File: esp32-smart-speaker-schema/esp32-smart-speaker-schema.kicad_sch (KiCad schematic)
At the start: 19 parts, among them J1 USB_C_Receptacle_USB2.0_14P, SW1 PWR_BTN, SW2 MODE_BTN, SW3 PREV_BTN, SW4 NXT_BTN, SW5 PAUS-BTN, U2 MAX98357A

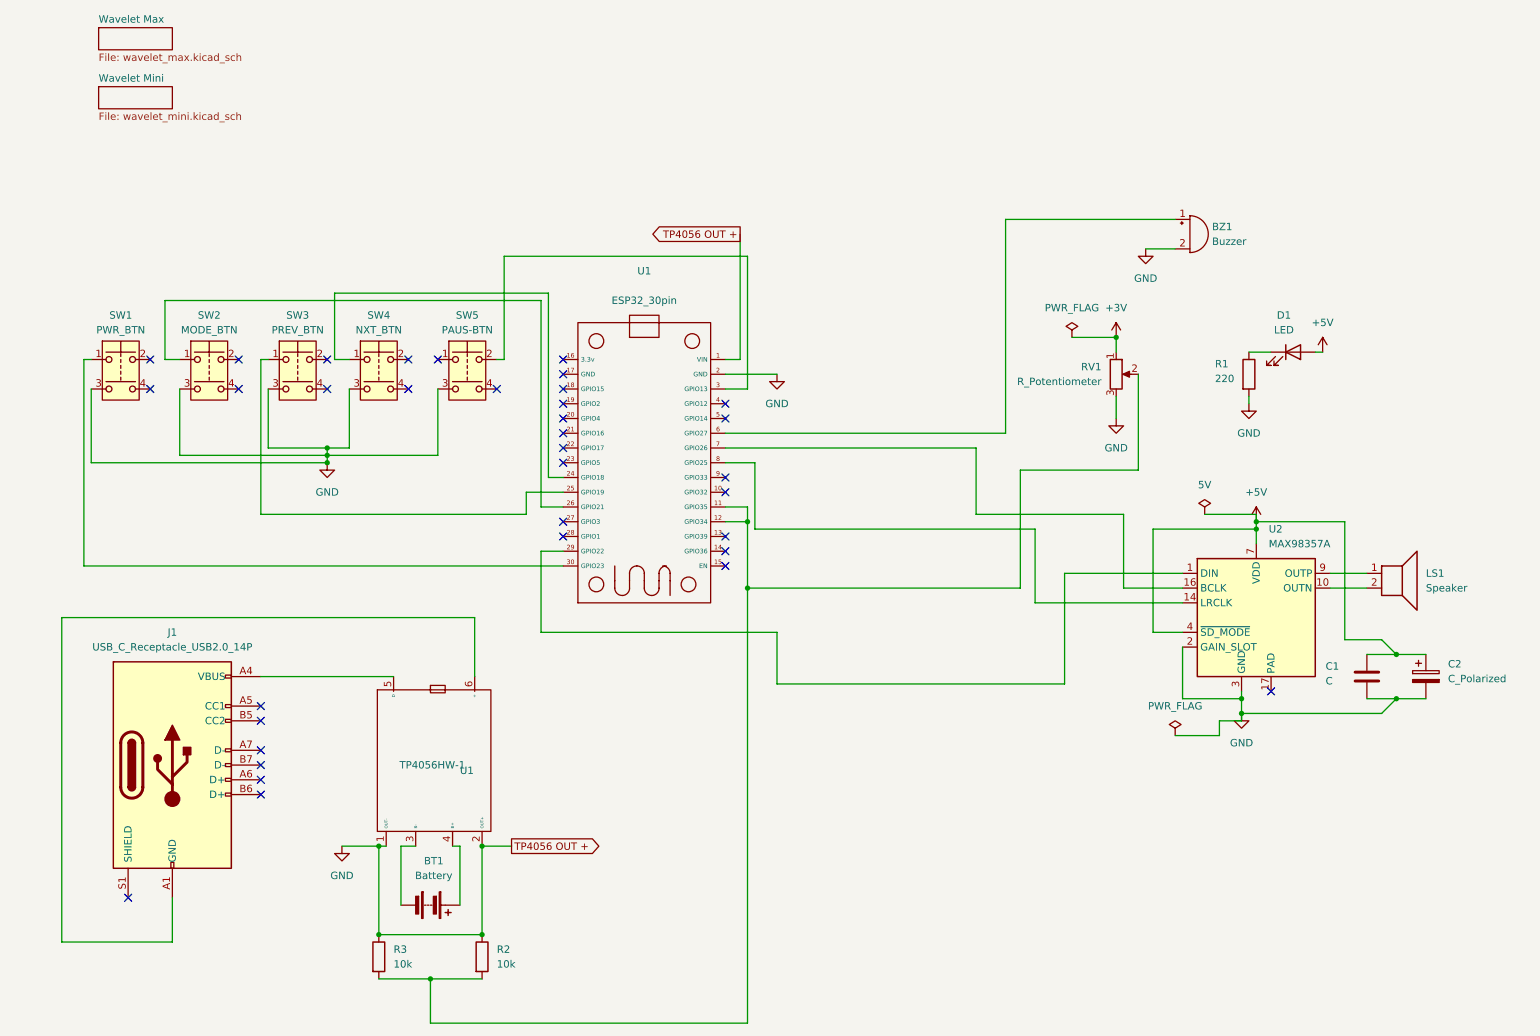
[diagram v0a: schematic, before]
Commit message: Started developing backend for wavelet mini
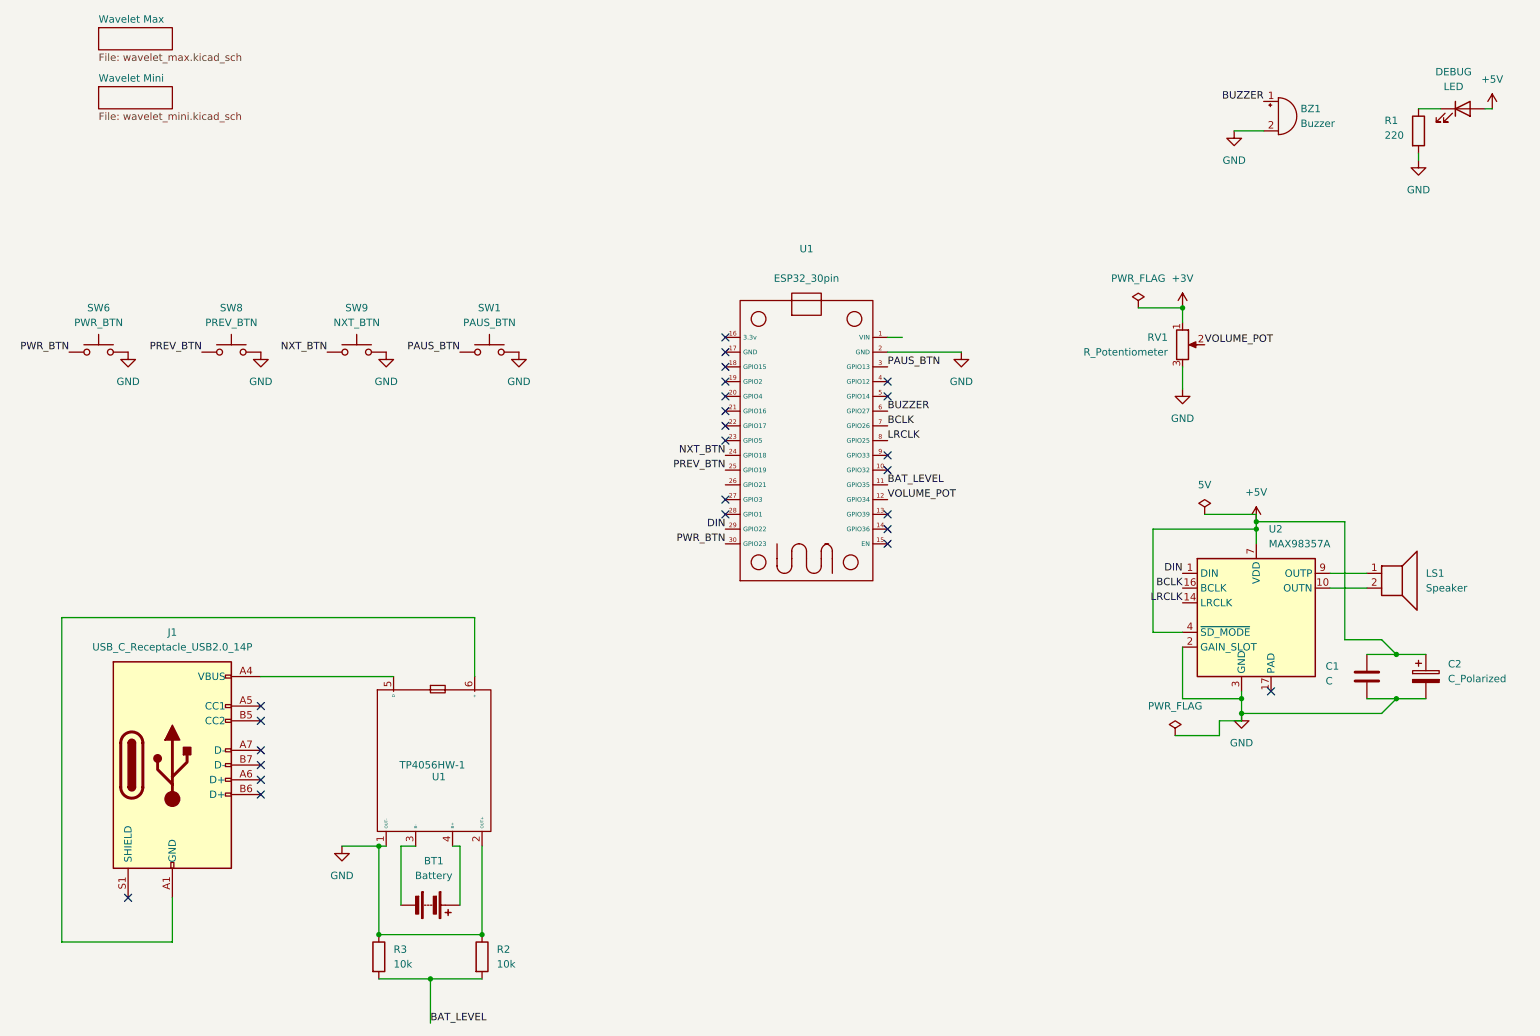
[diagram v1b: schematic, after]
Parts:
- removed SW1: PWR_BTN, symbol Switch:SW_Push_Dual
- removed SW2: MODE_BTN, symbol Switch:SW_Push_Dual
- removed SW3: PREV_BTN, symbol Switch:SW_Push_Dual
- removed SW4: NXT_BTN, symbol Switch:SW_Push_Dual
- removed SW5: PAUS-BTN, symbol Switch:SW_Push_Dual
- added SW1: PAUS_BTN, symbol Switch:SW_Push
- added SW6: PWR_BTN, symbol Switch:SW_Push
- added SW8: PREV_BTN, symbol Switch:SW_Push
- added SW9: NXT_BTN, symbol Switch:SW_Push
- renumbered D1 to DEBUG
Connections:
- net GND: now also SW1.2, SW6.2, SW8.2, SW9.2; no longer U1.1 (VIN)
- net BUZZER: now reaches BZ1.1 (+), U1.6 (GPIO27)
- net PAUS_BTN: now reaches U1.3 (GPIO13)
- net PAUS_BTN: now also SW1.1
- net BAT_LEVEL: now reaches R2.2, R3.2, U1.11 (GPIO35)
- net BAT_LEVEL: no longer RV1.2, U1.12 (GPIO34)
- net NXT_BTN: now reaches U1.24 (GPIO18)
- net NXT_BTN: now also SW9.1
- net PREV_BTN: now reaches U1.25 (GPIO19)
- net PREV_BTN: now also SW8.1
- net DIN: now reaches U1.29 (GPIO22), U2.1 (DIN)
- net PWR_BTN: now reaches U1.30 (GPIO23)
- net PWR_BTN: now also SW6.1
- net BCLK: now reaches U1.7 (GPIO26), U2.16 (BCLK)
- net LRCLK: now reaches U1.8 (GPIO25), U2.14 (LRCLK)
- new net VOLUME_POT: RV1.2, U1.12 (GPIO34)
- no-connect marks 35 -> 25
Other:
- moved on the sheet: BZ1, DEBUG, R1, RV1, U1
